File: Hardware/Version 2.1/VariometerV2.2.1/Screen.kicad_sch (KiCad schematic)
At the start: 20 parts, among them J4 FFC24/0.5MM, Q3 AO3400A

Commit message: Working on PCB
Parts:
- Q3: footprint (none) -> Package_TO_SOT_SMD:SOT-23
- R35: footprint (none) -> Resistor_SMD:R_0603_1608Metric
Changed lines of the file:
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@@
       (effects (font (size 1.27 1.27)))
     )
-    (property "Footprint" "" (at 83.82 85.09 0)
+    (property "Footprint" "Resistor_SMD:R_0603_1608Metric" (at 83.82 85.09 0)
       (effects (font (size 1.27 1.27)) hide)
     )
@@
       (effects (font (size 1.27 1.27)) (justify left))
     )
-    (property "Footprint" "" (at 106.68 83.185 0)
+    (property "Footprint" "Package_TO_SOT_SMD:SOT-23" (at 106.68 83.185 0)
       (effects (font (size 1.27 1.27) italic) (justify left) hide)
     )

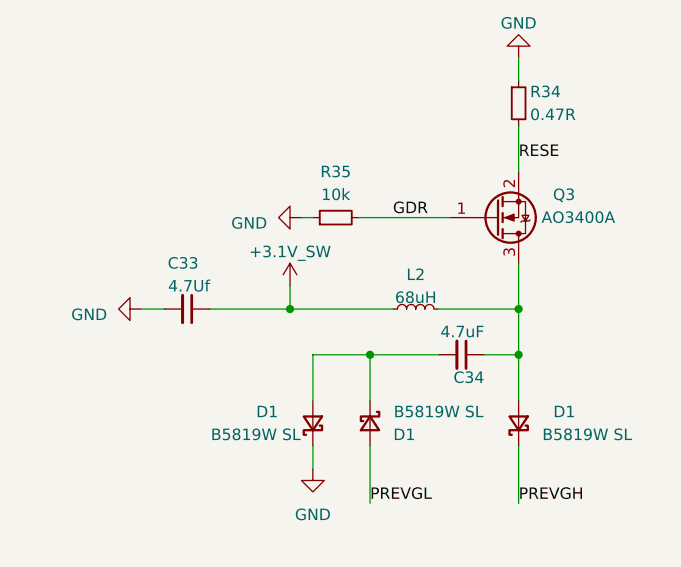
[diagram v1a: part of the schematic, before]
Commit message: PCB
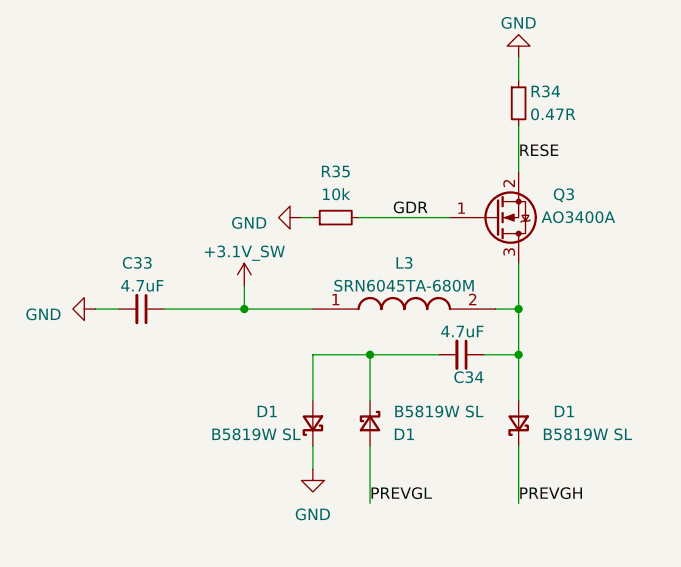
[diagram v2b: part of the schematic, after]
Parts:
- removed L2: 68uH, symbol Device:L_Small
- added L3: SRN6045TA-680M, MainLibrary:SRN6045TA, symbol Main_LibraryVario:SRN6045TA-680M
- C23, C24, C25, C26, C27, C28, C29, C31, C32: LCSC Part (none) -> C52923
- C30: LCSC Part (none) -> C19702
- C33: value 4.7Uf -> 4.7uF; LCSC Part (none) -> C19666
- C34: LCSC Part (none) -> C19666
- D1: JLCPCB Part # C8598 -> (none); LCSC Part (none) -> C8598
- J4: LCSC Part (none) -> C202112
- Q3: JLCPCB Part # C20917 -> (none); LCSC Part (none) -> C20917
- R34: footprint (none) -> Resistor_SMD:R_0805_2012Metric
- R35: LCSC Part (none) -> C25804
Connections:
- net +3.1V_SW: now also L3.1
- net at C34.1, D1.2 (A), Q3.3 (D): now also L3.2
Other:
- moved on the sheet: C33
